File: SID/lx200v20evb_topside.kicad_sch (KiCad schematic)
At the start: 0 parts

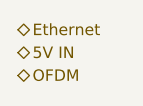
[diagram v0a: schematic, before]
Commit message: Feat(SID): basically complete
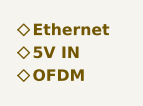
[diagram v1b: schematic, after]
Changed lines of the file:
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@@
-(kicad_sch (version 20230819) (generator eeschema)
-  (paper "A4")
-  (hierarchical_label "5V IN" (shape bidirectional) (at 102.87 86.36 0) (fields_autoplaced)
-    (effects (font (size 1.27 1.27)) (justify left))
-  )
-  (hierarchical_label "Ethernet" (shape bidirectional) (at 102.87 83.82 0) (fields_autoplaced)
-    (effects (font (size 1.27 1.27)) (justify left))
-  )
-  (hierarchical_label "OFDM" (shape bidirectional) (at 102.87 88.9 0) (fields_autoplaced)
-    (effects (font (size 1.27 1.27)) (justify left))
-  )
+(kicad_sch
+	(version 20240101)
+	(generator "eeschema")
+	(generator_version "8.99")
+	(paper "A4")
+	(hierarchical_label "5V IN"
+		(shape bidirectional)
+		(at 102.87 86.36 0)
+		(fields_autoplaced yes)
+		(effects
+			(font
+				(face "JetBrains Mono")
+				(size 1.27 1.27)
+				(thickness 0.254)
+				(bold yes)
+			)
+			(justify left)
+		)
+	)
+	(hierarchical_label "Ethernet"
+		(shape bidirectional)
+		(at 102.87 83.82 0)
+		(fields_autoplaced yes)
+		(effects
+			(font
+				(face "JetBrains Mono")
+				(size 1.27 1.27)
+				(thickness 0.254)
+				(bold yes)
+			)
+			(justify left)
+		)
+	)
+	(hierarchical_label "OFDM"
+		(shape bidirectional)
+		(at 102.87 88.9 0)
+		(fields_autoplaced yes)
+		(effects
+			(font
+				(face "JetBrains Mono")
+				(size 1.27 1.27)
+				(thickness 0.254)
+				(bold yes)
+			)
+			(justify left)
+		)
+	)
 )
